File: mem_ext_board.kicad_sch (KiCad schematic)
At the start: 13 parts, among them J1 Conn_02x05_Odd_Even, J2 Conn_02x02_Odd_Even, J3 Conn_02x16_Row_Letter_First, U1 74LS30, U2 AS6C1008-xxT, U4 74LS86

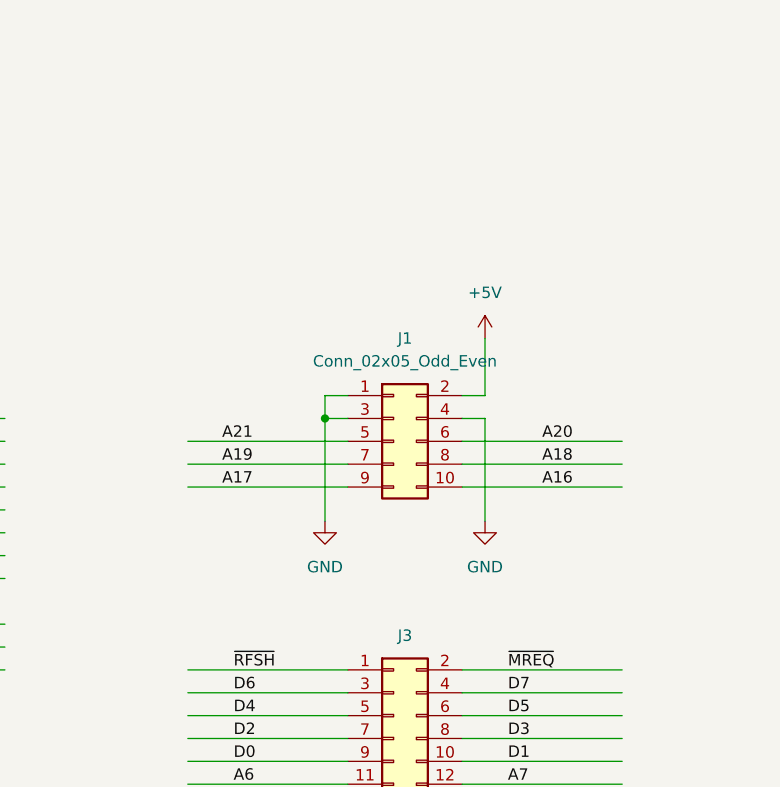
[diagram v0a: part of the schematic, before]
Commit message: Updated board to hopefully final shape
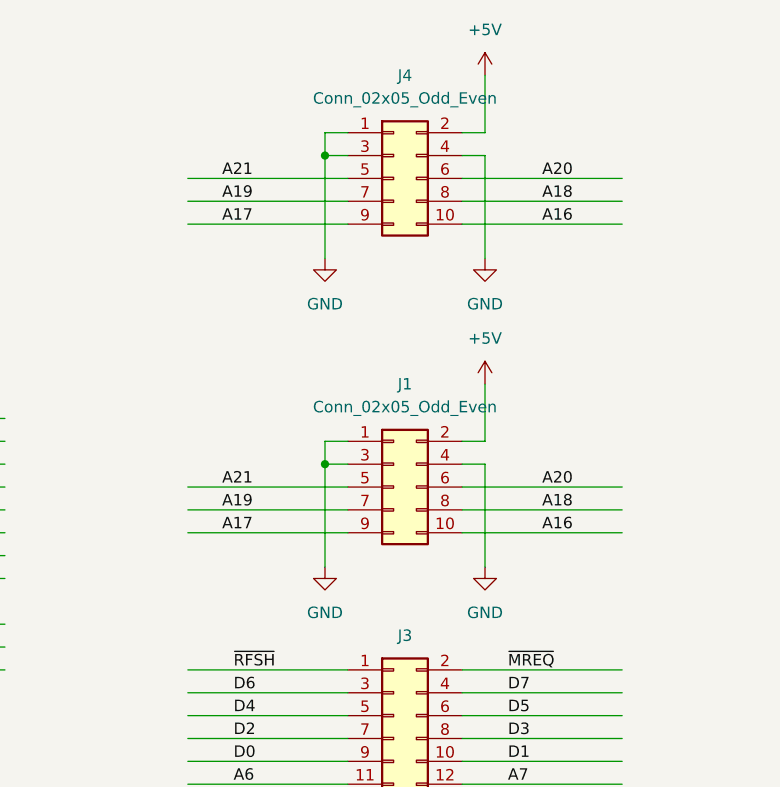
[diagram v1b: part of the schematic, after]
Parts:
- added J4: Conn_02x05_Odd_Even, Connector_PinSocket_2.54mm:PinSocket_2x05_P2.54mm_Vertical, symbol Connector_Generic:Conn_02x05_Odd_Even
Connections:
- net +5V: now also J4.2 (Pin_2)
- net A16: now also J4.10 (Pin_10)
- net A17: now also J4.9 (Pin_9)
- net A18: now also J4.8 (Pin_8)
- net A19: now also J4.7 (Pin_7)
- net A20: now also J4.6 (Pin_6)
- net A21: now also J4.5 (Pin_5)
- net GND: now also J4.1 (Pin_1), J4.3 (Pin_3), J4.4 (Pin_4)
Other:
- moved on the sheet: J1
